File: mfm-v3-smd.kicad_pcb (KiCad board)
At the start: 2 copper layers, 74.8 x 85.8 mm, 47 parts, among them J1 MFM Module-Left, J2 MFM Module-Right, J3 SMBUS Connector, J4 FTDI Connector, J5 ICSP Connector, J6 Antenna, J7 JST Jack, Q1 R.V. Protect, SW1 SW_VBAT, SW2 RESET, SW3 SW_LED_PWR, SW4 SW_LED_STAT, U1 MCP1703A-3302_SOT89, U2 LoRa_Radio, U3 ATmega1284P-AU, Y1 8MHz

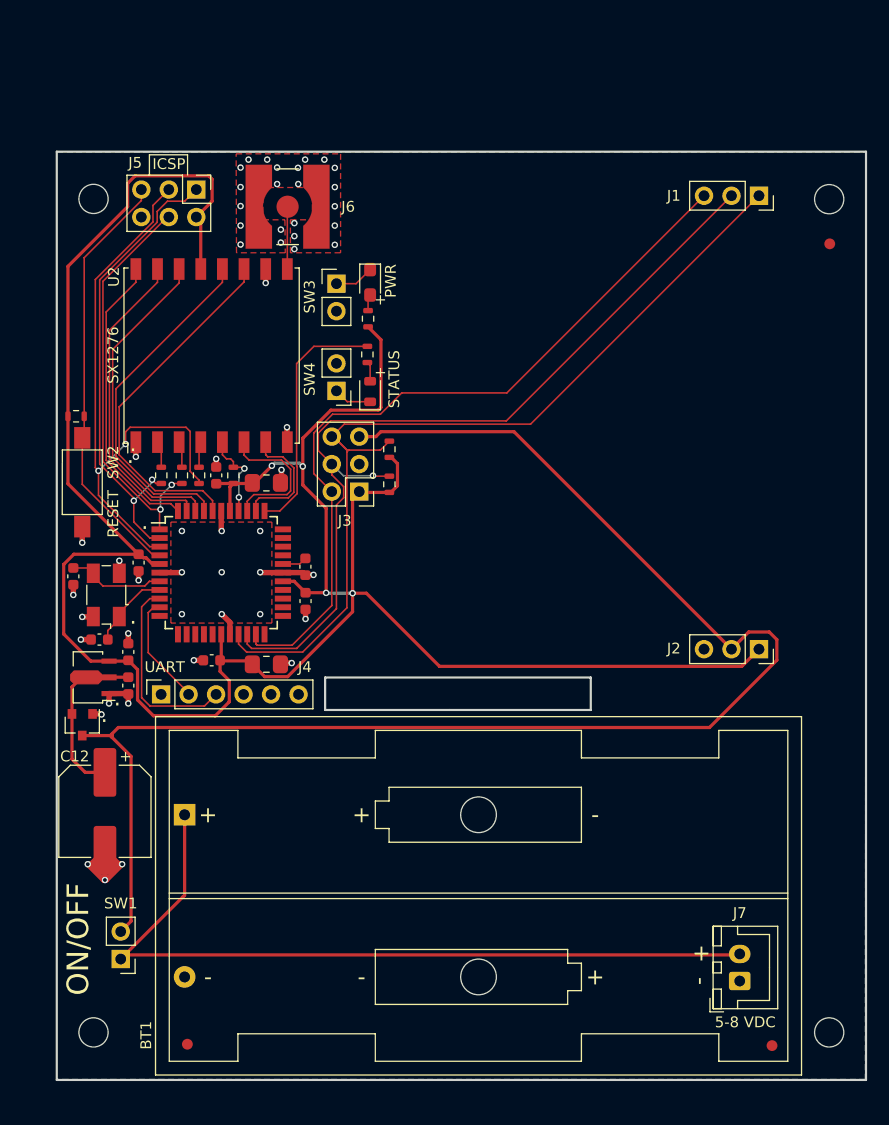
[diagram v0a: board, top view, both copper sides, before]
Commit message: initial setup of v3.7
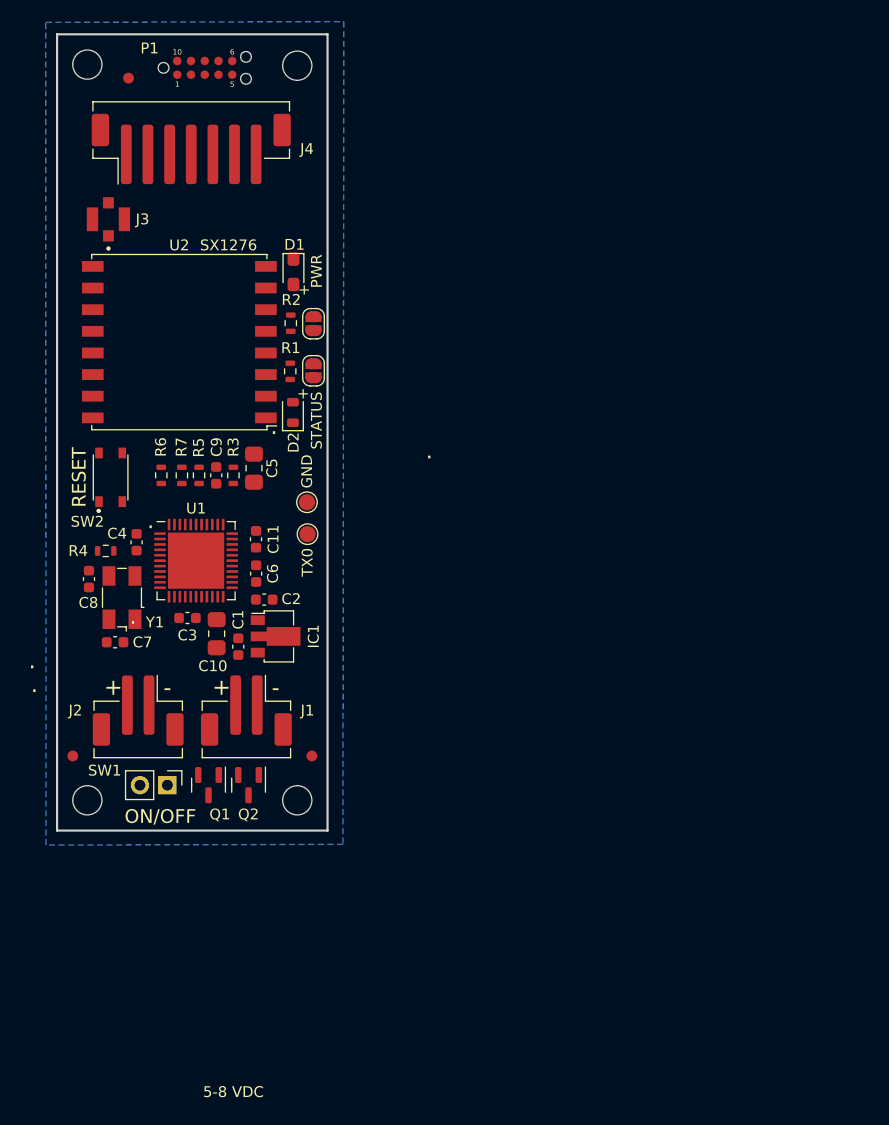
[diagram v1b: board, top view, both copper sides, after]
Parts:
- removed BT1: Battery, Battery:BatteryHolder_Keystone_2462_2xAA
- removed C12: 820uF 16v, Capacitor_SMD:C_Elec_8x10.2
- removed the J2 at (83.4, 125.0)
- removed the J3 at (46.4, 110.5)
- removed J5: ICSP Connector, Connector_PinHeader_2.54mm:PinHeader_2x03_P2.54mm_Vertical
- removed the R6 at (49.2, 109.8)
- removed R9: 4k7, custom_library_FP:R_0603_1608Metric_CRCW...C
- removed SW3: SW_LED_PWR, Connector_PinHeader_2.54mm:PinHeader_1x02_P2.54mm_Vertical
- removed SW4: SW_LED_STAT, Connector_PinHeader_2.54mm:PinHeader_1x02_P2.54mm_Vertical
- removed U3: ATmega1284P-AU, Package_QFP:TQFP-44_10x10mm_P0.8mm
- added IC1: AP7370-33Y, Package_TO_SOT_SMD:SOT-89-3, F.Cu at (38.7, 123.8)
- added JP1: SW_LED_PWR, Jumper:SolderJumper-2_P1.3mm_Open_RoundedPad1.0x1.5mm, F.Cu at (42.2, 95.0)
- added JP2: SW_LED_STAT, Jumper:SolderJumper-2_P1.3mm_Open_RoundedPad1.0x1.5mm, F.Cu at (42.2, 99.3)
- added P1: AVR-JTAG-10-TC2050(non-reversed), Tag-Connect_footprints:TC2050-IDC-NL, F.Cu at (32.1, 71.3)
- added Q2: R.V. Protect, Package_TO_SOT_SMD:SOT-23, F.Cu at (36.2, 137.6)
- added TP1: GND, TestPoint:TestPoint_Pad_D1.5mm, F.Cu at (41.6, 111.5)
- added TP2: TX0, TestPoint:TestPoint_Pad_D1.5mm, F.Cu at (41.6, 114.4)
- J1: value MFM Module-Left -> JST Jack; footprint custom_library_FP:MFM_Module_Board_P123 -> Connector_JST:JST_PH_B2B-PH-SM4-TB_1x02-1MP_P2.00mm_Vertical
- J2: renamed from J7; footprint Connector_JST:JST_XH_B2B-XH-A_1x02_P2.50mm_Vertical -> Connector_JST:JST_PH_B2B-PH-SM4-TB_1x02-1MP_P2.00mm_Vertical
- J3: renamed from J6; footprint custom_library_FP:LINX_CONSMA001-SMD-G -> CONMHF1-SMD-G-T:LINX_CONMHF1-SMD-G-T
- J4: value FTDI Connector -> MFM Module connector; footprint Connector_PinSocket_2.54mm:PinSocket_1x06_P2.54mm_Vertical -> Connector_JST:JST_PH_B7B-PH-SM4-TB_1x07-1MP_P2.00mm_Vertical
- SW2: footprint custom_library_FP:SW_SPST_PTS636 -> PTS815-SJK-250-SMTR-LFS:PTS815SJK250SMTRLFS
- U1: value MCP1703A-3302_SOT89 -> ATmega1284P-M; footprint custom_library_FP:SOT-89-3_MCP1703 -> Package_DFN_QFN:QFN-44-1EP_7x7mm_P0.5mm_EP5.2x5.2mm
- moved J1 67.1 mm to (36.0, 130.7), turned to 180 degrees
- moved FID2 66.6 mm to (25.1, 72.2)
- moved J2 61.0 mm to (26.0, 130.7), turned to 180 degrees
- moved H2 53.6 mm to (40.7, 139.0)
- moved H1 50.7 mm to (40.7, 71.1)
- moved J4 50.5 mm to (30.9, 78.8), turned to 0 degrees
- moved FID3 50.3 mm to (42.0, 134.9)
- moved FID1 28.7 mm to (19.9, 134.9)
- moved H4 21.5 mm to (21.3, 139.0)
- moved SW1 16.6 mm to (28.7, 137.6), turned to -90 degrees
- moved J3 16.6 mm to (23.2, 85.3), turned to 180 degrees
- moved U1 14.5 mm to (31.4, 116.8), turned to 0 degrees
- moved C2 13.5 mm to (37.6, 120.5), turned to 180 degrees
- moved Q1 12.9 mm to (32.5, 137.6)
- moved R4 12.7 mm to (23.0, 115.9), turned to 0 degrees
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- renumbered R8 to R6
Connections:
- C1 pad 2: Net-(C1-Pad2) -> VBAT
- J1 pad 1: I2C_SCL -> GND
- J1 pad 2: I2C_SDA -> /Bat_in_2
- J2 pad 2: Net-(BT1-Pad1) -> /Bat_in_1
- J4 pad 1: (no net) -> +3V3
- J4 pad 2: AVR_TX0 -> VBAT
- J4 pad 3: AVR_RX0 -> I2C_SCL
- J4 pad 4: (no net) -> GND
- J4 pad 5: (no net) -> SMBALERT
- J4 pad 6: GND -> I2C_SDA
- Q1 pad 2: Net-(C1-Pad2) -> Net-(Q1-Pad2)
- Q1 pad 3: VBAT -> /Bat_in_1
- SW1 pad 1: Net-(BT1-Pad1) -> Net-(Q1-Pad2)
- U1 pad 1: GND -> AVR_MOSI
- U1 pad 2: Net-(C1-Pad2) -> AVR_MISO
- U1 pad 3: +3V3 -> AVR_SCK
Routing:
- net +3V3: track 225.0 -> 0.00 mm, vias 4 -> 0
- net VBAT: track 136.7 -> 0.00 mm
- net I2C_SCL: track 84.4 -> 0.00 mm
- net I2C_SDA: track 81.4 -> 0.00 mm, vias 1 -> 0
- net Net-(BT1-Pad1): track 73.9 -> 0.00 mm
- net SMBALERT: track 71.3 -> 0.00 mm
- net AVR_SCK: track 54.9 -> 0.00 mm, vias 2 -> 0
- net GND: track 46.1 -> 0.00 mm, vias 54 -> 0
- net AVR_MISO: track 43.3 -> 0.00 mm, vias 2 -> 0
- net NRST: track 39.5 -> 0.00 mm
- net AVR_MOSI: track 38.3 -> 0.00 mm, vias 2 -> 0
- net RADIO_DIO3: track 33.3 -> 0.00 mm
- net RADIO_DIO4: track 32.1 -> 0.00 mm
- net RADIO_DIO0: track 30.2 -> 0.00 mm
- net RADIO_DIO1: track 29.0 -> 0.00 mm
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- removed copper zone on F.Cu, net GND
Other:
- board size 74.8 x 85.8 mm -> 25 x 73.6 mm
- board text added: "MFM Brain board v3.7 2022-02-18 Senwize B.V."
- board text removed: "3V3"
- board text removed: "GND"
- board text removed: "ICSP"
- board text removed: "MCU RX0"
- board text removed: "MCU TX0"
- board text removed: "MFM Brain board v3.6 2021-10-23 Senwize B.V."
- board text removed: "SCL"
- board text removed: "SDA"
- board text removed: "SMBA"
- board text removed: "UART"
- board text removed: "VBAT"
